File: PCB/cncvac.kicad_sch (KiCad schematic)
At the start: 34 parts, among them J1 AVR-ISP-6, J2 24VAC, SW1 SW_SPST, U1 ATtiny841-SS, U2 MICRF112YMM, U3 LTV-357T, Y1 13.56MHz, Y2 8MHz

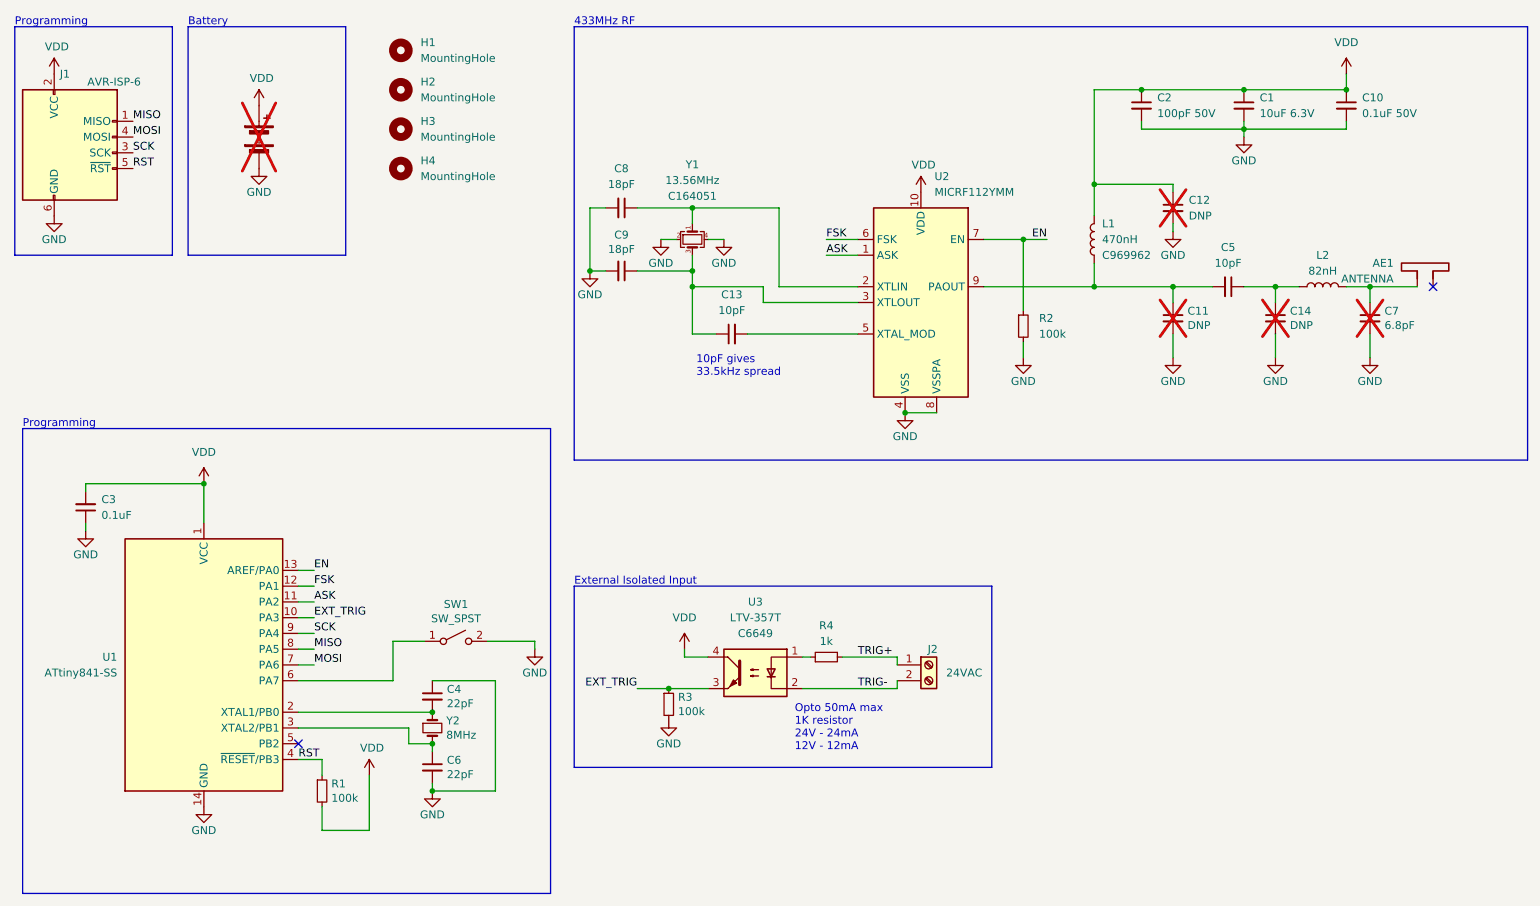
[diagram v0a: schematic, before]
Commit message: givver
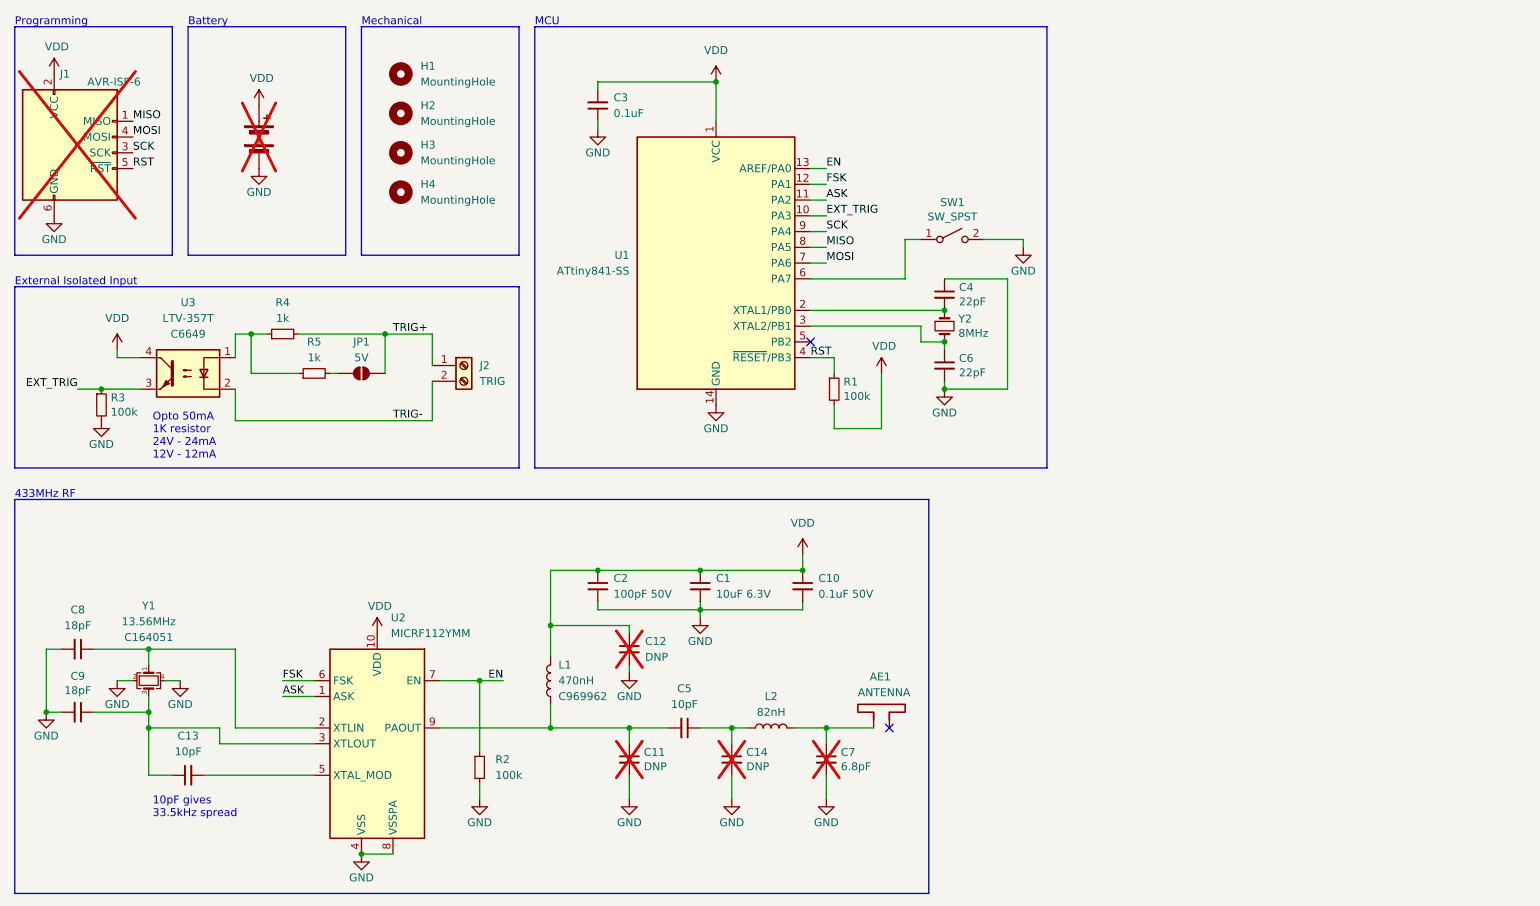
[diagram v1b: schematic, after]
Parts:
- added JP1: 5V, Jumper:SolderJumper-2_P1.3mm_Open_RoundedPad1.0x1.5mm, symbol Jumper:SolderJumper_2_Open
- added R5: 1k, Resistor_SMD:R_0402_1005Metric, symbol Device:R_Small
- J1: now not fitted
- J2: value 24VAC -> TRIG
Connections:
- net TRIG+: now also JP1.2 (B)
- net at R4.1, U3.1: now also R5.1
- new net: JP1.1 (A), R5.2
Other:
- note added: "MCU"
- note added: "Mechanical"
- note added: "Opto 50mA 1K resistor 24V - 24mA 12V - 12mA"
- note removed: "Opto 50mA max 1K resistor 24V - 24mA 12V - 12mA"
- moved on the sheet: AE1, C1, C10, C11, C12, C13, C14, C2, C3, C4, C5, C6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
